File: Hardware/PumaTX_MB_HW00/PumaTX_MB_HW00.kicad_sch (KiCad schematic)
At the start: 120 parts, among them J100 FH12A-26S-0.5SH_55_, J101 FH12-12S-0.5SH_55_, J102 500334-0160, J103 500334-0160, J104 692122030100, J105 53398-0667, J400 U.FL-R-SMT-1_40_, J410 U.FL-R-SMT-1_40_, M130 Motor_DC, M140 Fan, Q130 ZXMN3B01F, Q140 ZXMN3B01F, Q200 UMH3NTN, Q201 UMH3NTN, U200 CP2105-F01-GMR, U300 ESP32-PICO-D4, U400 ESP32-PICO-D4, U402 E28-2G4M27S, U410 SX1280, U500 BQ24075RGTR, U510 MIC5528-3.3YMT-T5, U520 MIC5528-3.3YMT-T5, U530 MIC5528-3.3YMT-T5, Y410 NX2016SA-52MHZ-EXS00A-CS06016

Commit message: and on and on and on... It is getting harder
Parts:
- C201: footprint Capacitor_SMD:C_0402_1005Metric -> Capacitor_SMD:C_0603_1608Metric
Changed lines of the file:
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@@
       (effects (font (size 1.27 1.27)) (justify left))
     )
-    (property "Footprint" "Capacitor_SMD:C_0402_1005Metric" (id 2) (at 376.8852 88.9 0)
+    (property "Footprint" "Capacitor_SMD:C_0603_1608Metric" (id 2) (at 376.8852 88.9 0)
       (effects (font (size 1.27 1.27)) hide)
     )
@@
     )
     (path "/992d47c1-3d77-49c3-9a69-0e410ebfa256"
-      (reference "C201") (unit 1) (value "100n") (footprint "Capacitor_SMD:C_0402_1005Metric")
+      (reference "C201") (unit 1) (value "100n") (footprint "Capacitor_SMD:C_0603_1608Metric")
     )
     (path "/ece295b9-b570-401a-92a8-013600552bb1"

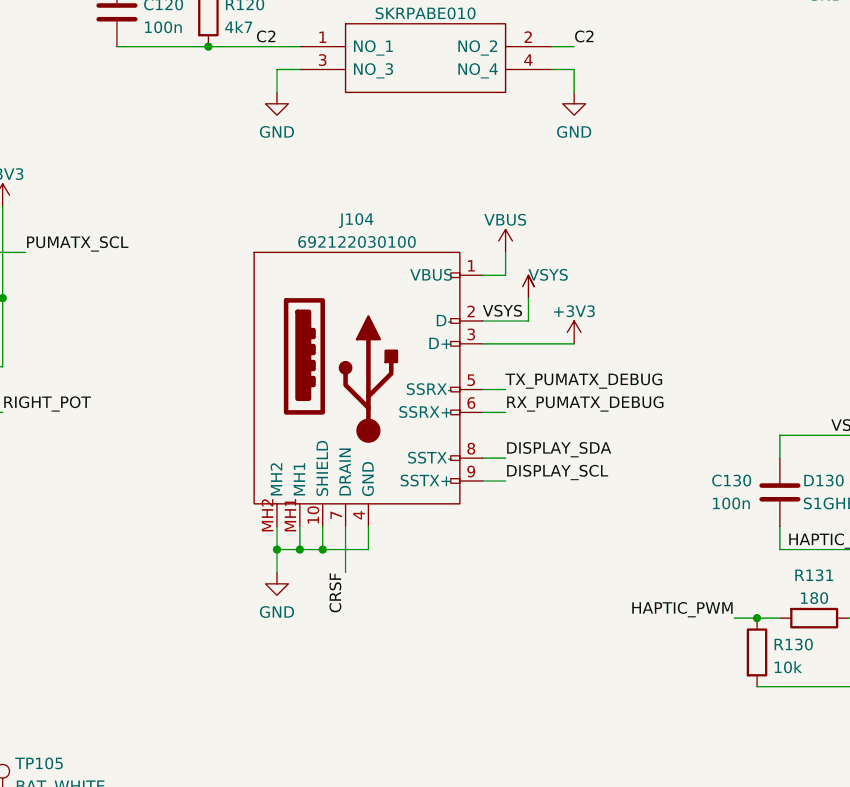
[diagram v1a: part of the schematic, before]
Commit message: Wow its gonna be complicated
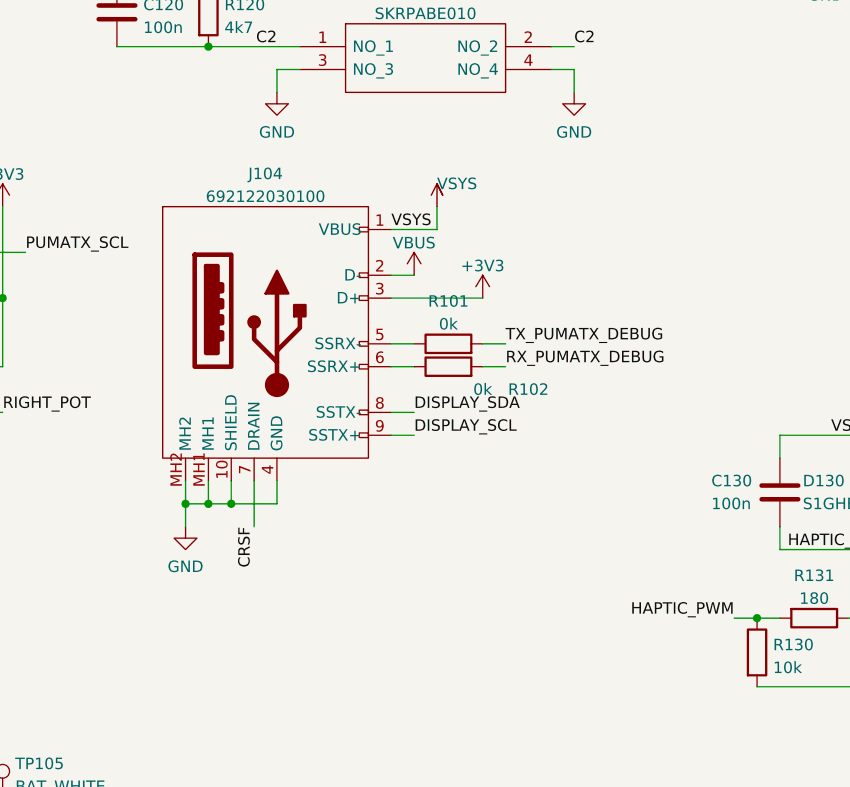
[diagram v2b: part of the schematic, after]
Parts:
- added R101, R102: 0k, Capacitor_SMD:C_0402_1005Metric, symbol Component_lib:R
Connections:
- net RX_PUMATX_DEBUG: now also R102.2; no longer J104.6 (SSRX+)
- net TX_PUMATX_DEBUG: now also R101.2; no longer J104.5 (SSRX-)
- net VBUS: now also J104.2 (D-); no longer J104.1 (VBUS)
- net VSYS: now also J104.1 (VBUS); no longer J104.2 (D-)
- new net: J104.5 (SSRX-), R101.1
- new net: J104.6 (SSRX+), R102.1
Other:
- moved on the sheet: J104
